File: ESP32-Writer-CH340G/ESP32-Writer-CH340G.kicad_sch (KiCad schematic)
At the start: 27 parts, among them J1 ESP-Prog-ProgramCOM-SEND, J2 USB2.0_C, J3 UART-OUTPUT, J4 USB2.0_C, Q1 2N7002, Q2 2N7002, U1 AMS1117-3.3, U2 CH340G, Y1 12M

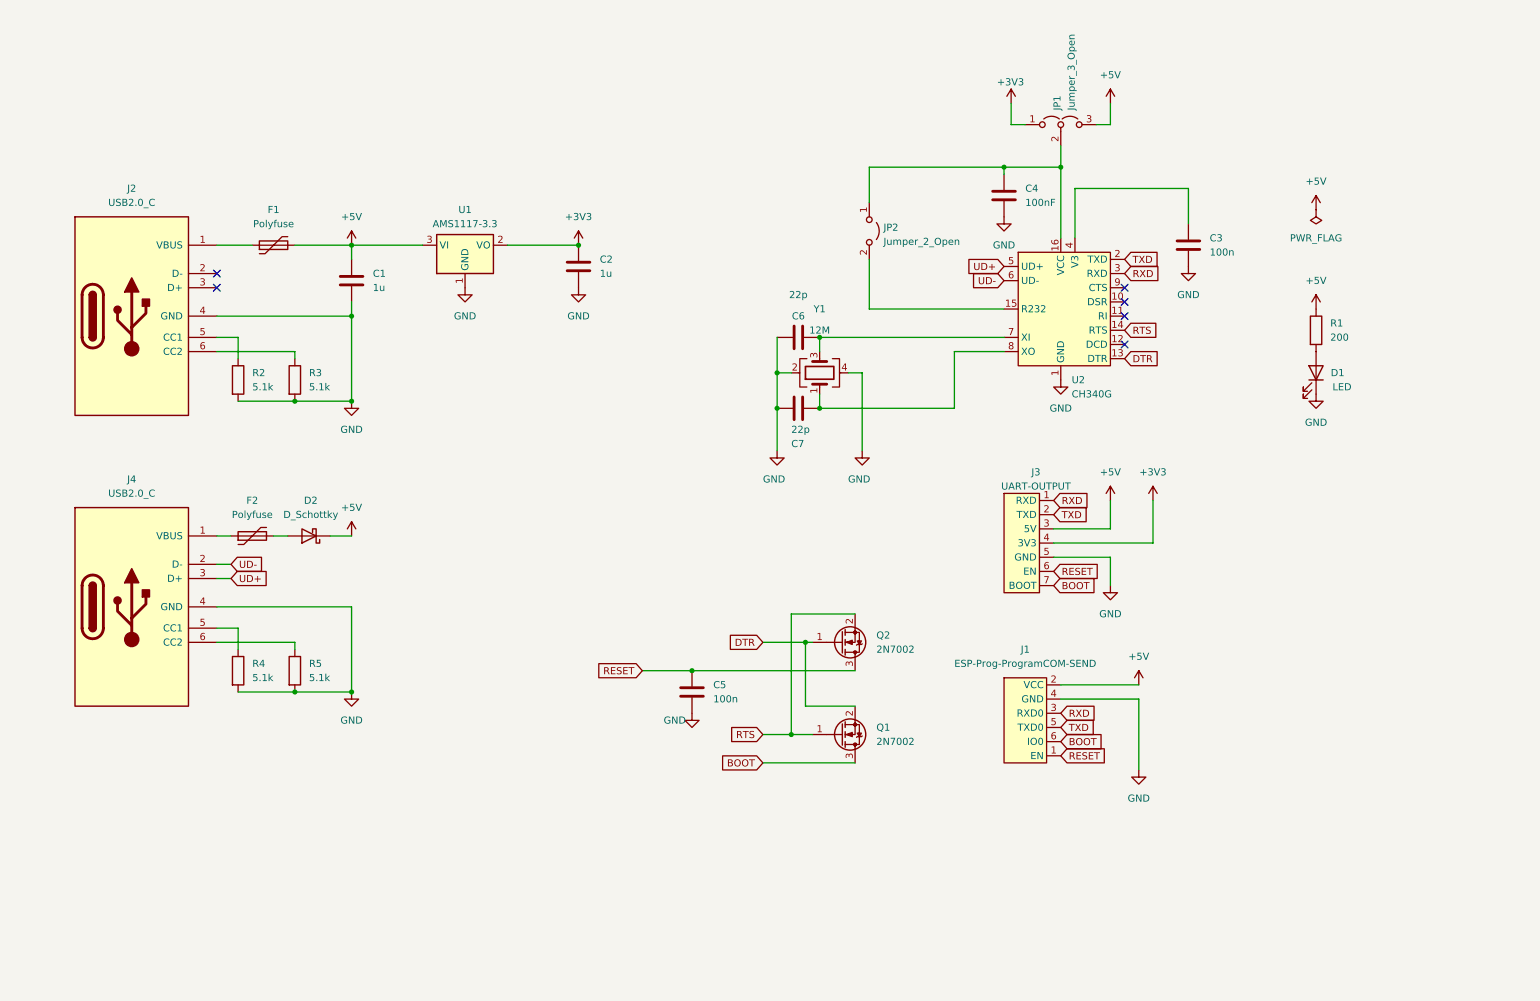
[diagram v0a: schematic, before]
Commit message: esp32-writer/v3.0.0
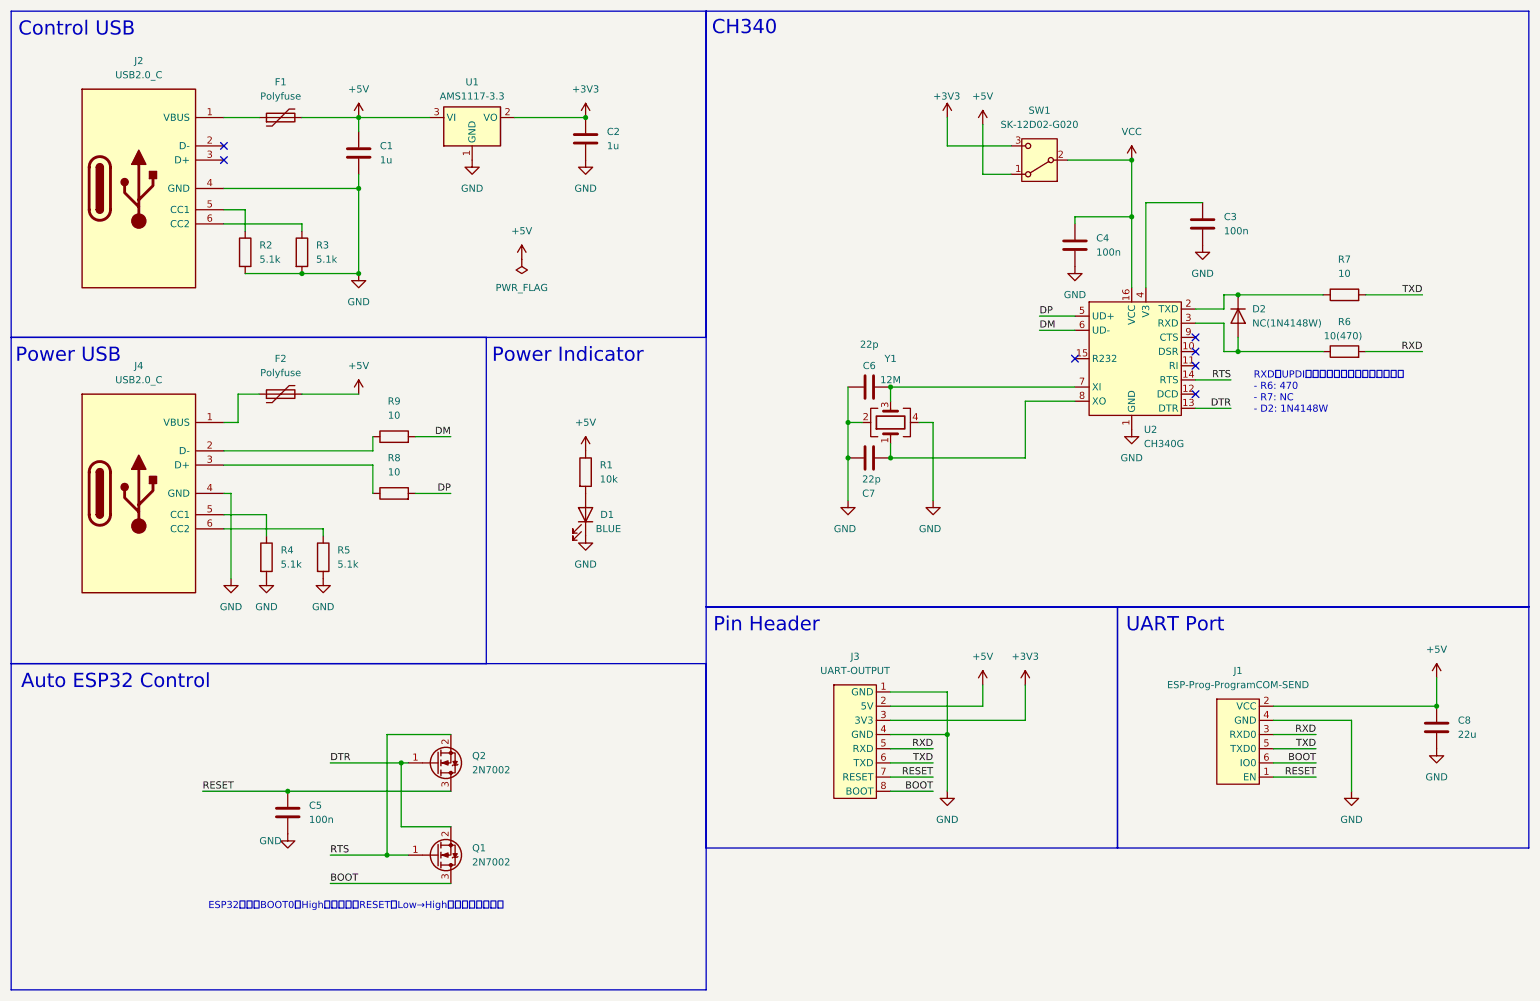
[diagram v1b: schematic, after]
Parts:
- removed D2: D_Schottky, $74th:D_SMA, symbol Device:D_Schottky
- removed JP1: Jumper_3_Open, Jumper:SolderJumper-3_P1.3mm_Open_RoundedPad1.0x1.5mm_NumberLabels, symbol Jumper:Jumper_3_Open
- removed JP2: Jumper_2_Open, Jumper:SolderJumper-2_P1.3mm_Open_RoundedPad1.0x1.5mm, symbol Jumper:Jumper_2_Open
- added C8: 22u, 74th:Capacitor_0805_2012, symbol Device:C
- added D2: NC(1N4148W), 74th:Package_SOD23_Diode, symbol Device:D
- added R6: 10(470), $74th:Register_0805_2012, symbol Device:R
- added R7: 10, $74th:Register_0805_2012, symbol Device:R
- added R8, R9: 10, 74th:Register_0805_2012, symbol Device:R
- added SW1: SK-12D02-G020, 74th:Switch_Slide_SK-12D02-G020, symbol 74th_Interface:SW_Slide
- C1, C2, C3, C5, C6, C7: footprint $74th:Capacitor_0805_2012 -> 74th:Capacitor_0805_2012
- C4: value 100nF -> 100n; footprint $74th:Capacitor_0805_2012 -> 74th:Capacitor_0805_2012
- D1: value LED -> BLUE; footprint $74th:LED_0805_2012Metric_Pad1.15x1.40mm_HandSolder -> 74th:LED_0805_2012
- F1, F2: footprint $74th:Fuse_1812_4532Metric_Pad1.30x3.40mm_HandSolder -> 74th:Package_Fuse_1812_4532m
- J1: symbol $74th:ESP-Prog-ProgramCOM-SEND -> 74th_Interface:ESP-Prog-ProgramCOM_SEND
- J2, J4: footprint $74th:USB-C-12-Pin-MidMount-ali-v5 -> 74th:Connector_USB-C-Receptacle_SMT_12-Pin_Simple; symbol esp32-dev-board:USB2.0_C -> 74th_Interface:USB_TypeC-2.0_Receptacle
- J3: footprint esp32-dev-board:UART -> 74th:PinOut_Pin_8; symbol esp32-dev-board:UART-OUTPUT-v2 -> $symbol:PinHeader
- R1: value 200 -> 10k; footprint $74th:Register_0805_2012 -> 74th:Register_0805_2012
- R2, R3, R4, R5: footprint $74th:Register_0805_2012 -> 74th:Register_0805_2012
- U2: footprint Package_SO:SOP-16_3.9x9.9mm_P1.27mm -> 74th:Package_SOIC-16_3.9x9.9mm_P1.27mm; symbol $74th:CH340G -> 74th_ApplicationIC:CH340G_USB-UART
- Y1: footprint $74th:Crystal_SMD_3225-4Pin_3.2x2.5mm_HandSoldering -> 74th:Crystal_SMD_3225-4Pin_3.2x2.5mm_HandSoldering
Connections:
- net +3V3: now also J3.3 (3V3), SW1.3 (C); no longer J3.4 (3V3)
- net +5V: now also F2.2, J3.2 (5V), C8.1, SW1.1 (A); no longer J3.3 (5V)
- net BOOT: now also J3.8 (BOOT); no longer J3.7 (BOOT)
- net GND: now also J3.1 (GND), J3.4 (GND), C8.2; no longer J3.5 (GND)
- net RESET: now also J3.7 (RESET); no longer J3.6 (EN)
- net RXD: now also J3.5 (RXD), R6.2; no longer J3.1 (RXD), U2.3 (RXD)
- net TXD: now also J3.6 (TXD), R7.2; no longer J3.2 (TXD), U2.2 (TXD)
- net VCC: now reaches C4.1, U2.16 (VCC)
- net VCC: now also SW1.2 (B)
- net UD+: no longer names the net of J4.3 (D+)
- net UD+: now also R8.1; no longer U2.5 (UD+)
- net UD-: no longer names the net of J4.2 (D-)
- net UD-: now also R9.1; no longer U2.6 (UD-)
- new net: D2.2 (A), R6.1, U2.3 (RXD)
- new net: D2.1 (K), R7.1, U2.2 (TXD)
- new net DM: R9.2, U2.6 (UD-)
- new net DP: R8.2, U2.5 (UD+)
- no-connect marks 6 -> 7
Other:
- note added: "Auto ESP32 Control"
- note added: "CH340"
- note added: "Control USB"
- note added: "ESP32では、BOOT0がHighの状態で、RESETがLow→Highになる必要がある"
- note added: "Pin Header"
- note added: "Power Indicator"
- note added: "Power USB"
- note added: "RXDをUPDI化する場合には以下に変更する - R6: 470 - R7: NC - D2: 1N4148W"
- note added: "UART Port"
- company: (none) -> Atsushi Morimoto (@74th)
- title: (none) -> ESP32-Writer
- moved on the sheet: C1, C2, C3, C4, C5, C6, C7, D1, F1, F2, J1, J2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
